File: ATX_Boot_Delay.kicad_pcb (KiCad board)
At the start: 2 copper layers, 74.9 x 17.1 mm, 14 parts, among them J1 ATX_FP, J2 ATX_FP, J3 SELECT, SW1 POWER, SW2 RESET

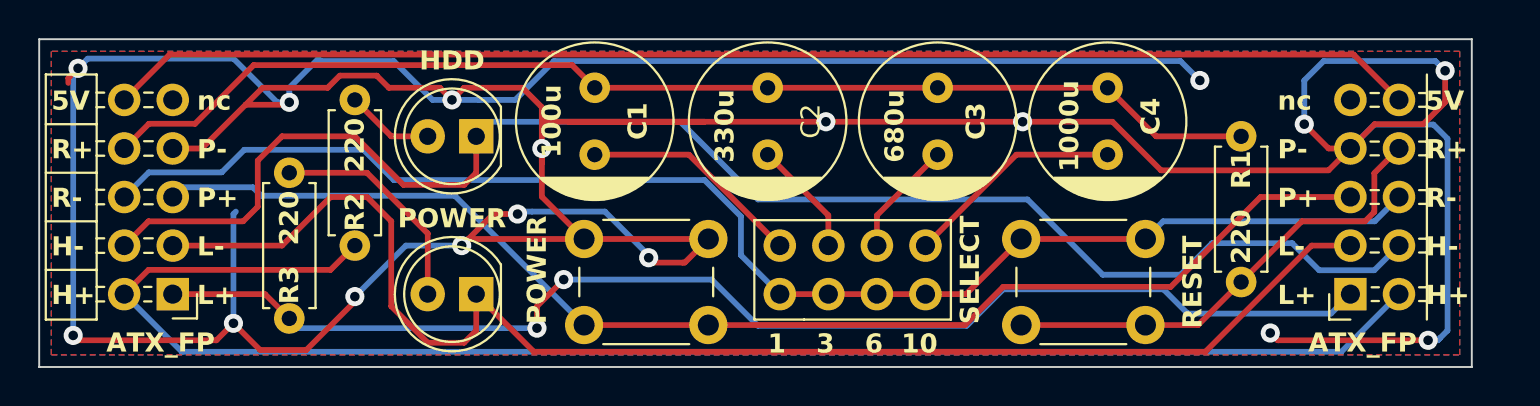
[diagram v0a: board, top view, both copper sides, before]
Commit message: Second Revision - v1.1
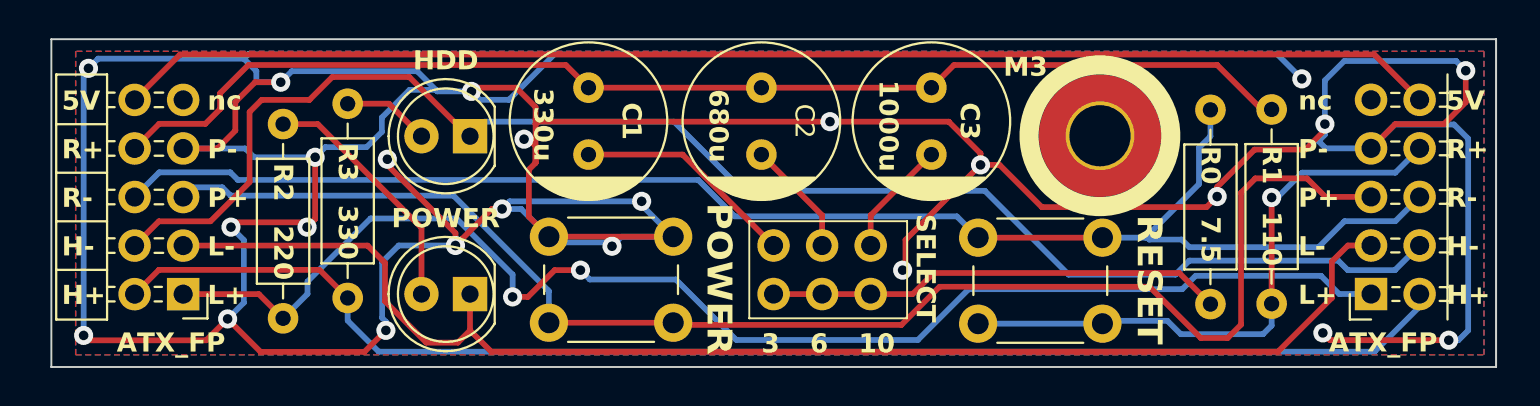
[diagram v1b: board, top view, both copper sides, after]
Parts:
- removed C4: 1000u, Capacitor_THT:C_Radial_D8.0mm_H11.5mm_P3.50mm
- added H1: M3, MountingHole:MountingHole_3.2mm_M3_Pad_TopOnly, F.Cu at (96.1, 38.1)
- added R0: 7.5, Resistor_THT:R_Axial_DIN0207_L6.3mm_D2.5mm_P10.16mm_Horizontal, F.Cu at (101.9, 36.7)
- C1: value 100u -> 330u
- C2: value 330u -> 680u
- C3: value 680u -> 1000u
- D1: value HDD -> POWER
- D2: value POWER -> HDD
- J3: footprint Connector_PinHeader_2.54mm:PinHeader_2x04_P2.54mm_Vertical -> Connector_PinHeader_2.54mm:PinHeader_2x03_P2.54mm_Vertical
- R1: value 220 -> 110; footprint Resistor_THT:R_Axial_DIN0207_L6.3mm_D2.5mm_P7.62mm_Horizontal -> Resistor_THT:R_Axial_DIN0207_L6.3mm_D2.5mm_P10.16mm_Horizontal
- R2: renamed from R3; footprint Resistor_THT:R_Axial_DIN0207_L6.3mm_D2.5mm_P7.62mm_Horizontal -> Resistor_THT:R_Axial_DIN0207_L6.3mm_D2.5mm_P10.16mm_Horizontal
- R3: renamed from R2; value 220 -> 330; footprint Resistor_THT:R_Axial_DIN0207_L6.3mm_D2.5mm_P7.62mm_Horizontal -> Resistor_THT:R_Axial_DIN0207_L6.3mm_D2.5mm_P10.16mm_Horizontal
- moved D2 8.27 mm to (63.2, 38.1)
- moved D1 8.26 mm to (63.2, 46.4)
- moved R3 2.77 mm to (56.8, 46.6)
- moved SW2 2.25 mm to (89.8, 43.4)
- moved R1 2.12 mm to (105.1, 36.7)
- moved SW1 1.84 mm to (67.3, 43.4)
- moved J2 1.08 mm to (110.3, 46.4)
- moved J1 0.55 mm to (48.2, 46.4)
- moved C1 0.33 mm to (69.4, 35.6)
- moved C2 0.33 mm to (78.4, 35.6)
- moved C3 0.33 mm to (87.3, 35.6)
- moved R2 0.33 mm to (53.4, 47.6)
- moved J3 0.33 mm to (79.0, 46.4)
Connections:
- D1 pad 1: HDD_LED- -> POWER_LED-
- D2 pad 1: POWER_LED- -> HDD_LED-
- J3 pad 1: RESET_SW- -> Net-(J3-Pin_1)
- J3 pad 3: RESET_SW- -> Net-(J3-Pin_1)
- J3 pad 5: RESET_SW- -> Net-(J3-Pin_1)
- R2 pad 2: Net-(D2-A) -> Net-(D1-A)
- R3 pad 2: Net-(D1-A) -> Net-(D2-A)
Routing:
- net POWER_SW-: track 267.0 -> 307.1 mm, vias 17 -> 24
- net Net-(J3-Pin_1): track 0.00 -> 24.0 mm
- net Net-(J3-Pin_8): track 11.5 -> 0.00 mm
- net HDD_LED+: track 82.3 -> 71.8 mm
- net POWER_SW+: track 67.6 -> 76.3 mm
- net Net-(D1-A): track 4.60 -> 13.0 mm
- net Net-(D2-A): track 11.7 -> 4.56 mm
- net EXT_RESET_SW+: track 24.8 -> 31.4 mm, vias 0 -> 1
- net POWER_LED+: track 66.8 -> 71.5 mm
- net RESET_SW-: track 74.5 -> 78.5 mm
- net POWER_LED-: track 74.1 -> 71.4 mm
- net RESET_SW+: track 61.8 -> 63.2 mm
- net +5V: track 68.6 -> 69.2 mm
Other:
- board size 74.9 x 17.1 mm -> 75.6 x 17.1 mm
- board text added: "ATX 9-Pin Front Panel Header In-Line Boot Delay"
